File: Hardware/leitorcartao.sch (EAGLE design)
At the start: 167 parts, among them IC1 TL084, IC2 TL084, Q1 BSH103, Q2 BC847ASMD, Q3 BC857ALT1SMD, Q4 BC847ALT1SMD, Q5 BC847ALT1SMD, Q6 BC847ALT1SMD, Q7 BC847ALT1SMD, U1 SAMD20E14A-AUT, U3 TLV1117-50CDCYR, U4 MFRC52202HN1, U5 LP2985-33DBVR, X1 ANTENA 125kHz, X2 MIFARE ANTENA

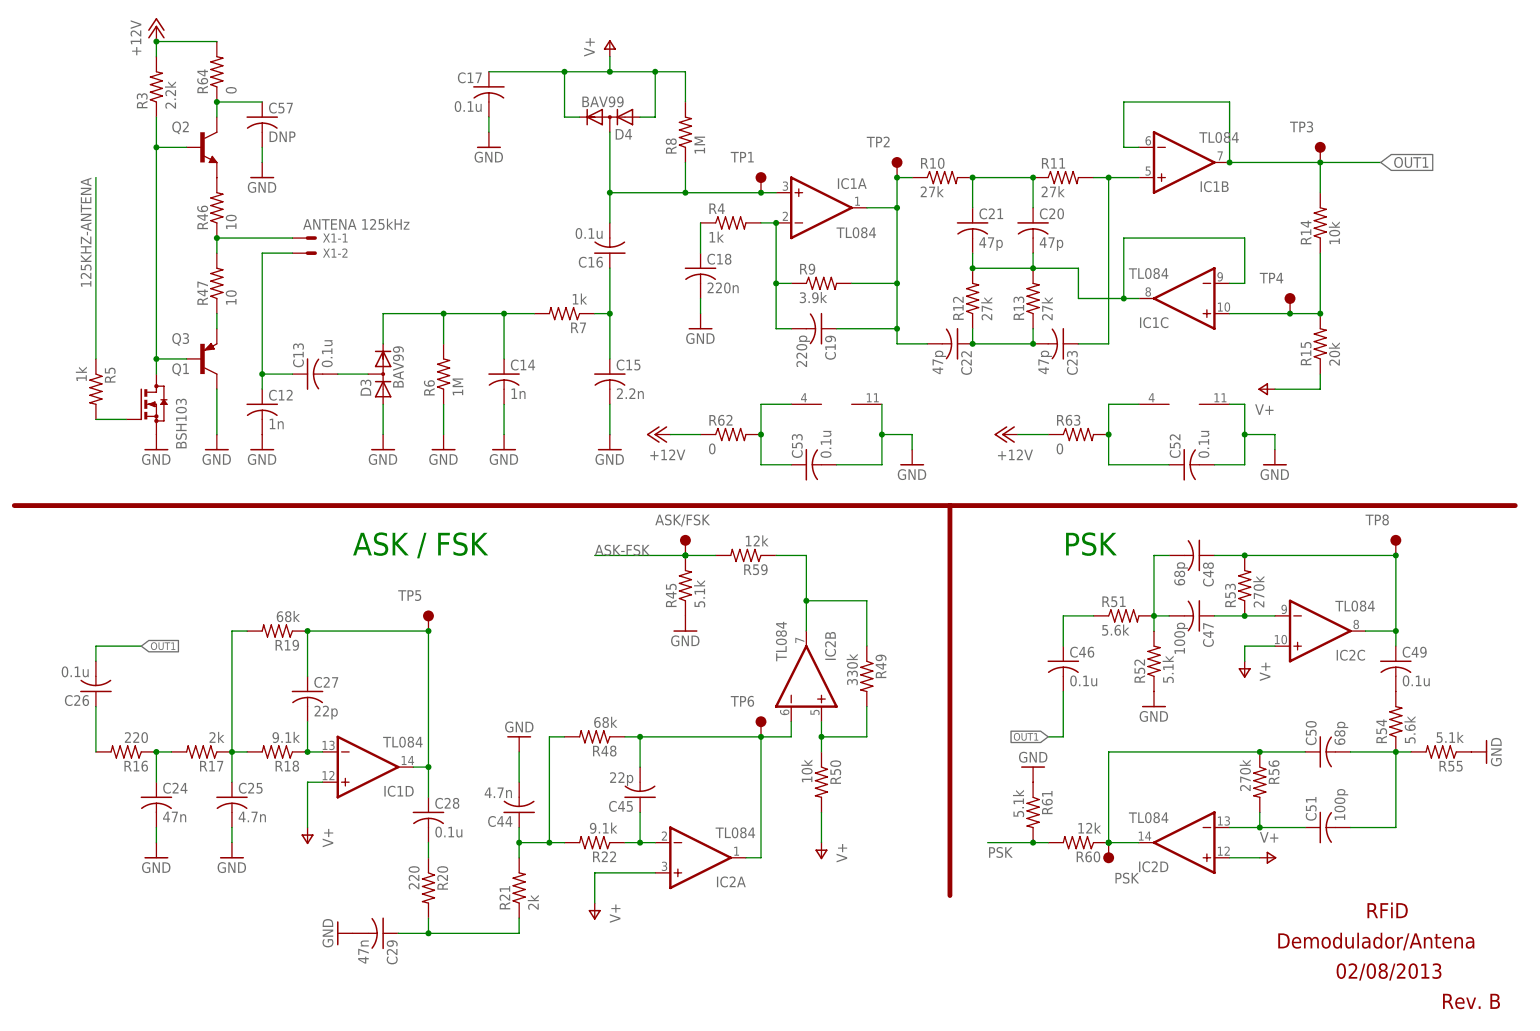
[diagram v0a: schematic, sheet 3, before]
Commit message: Início da versão 3.0
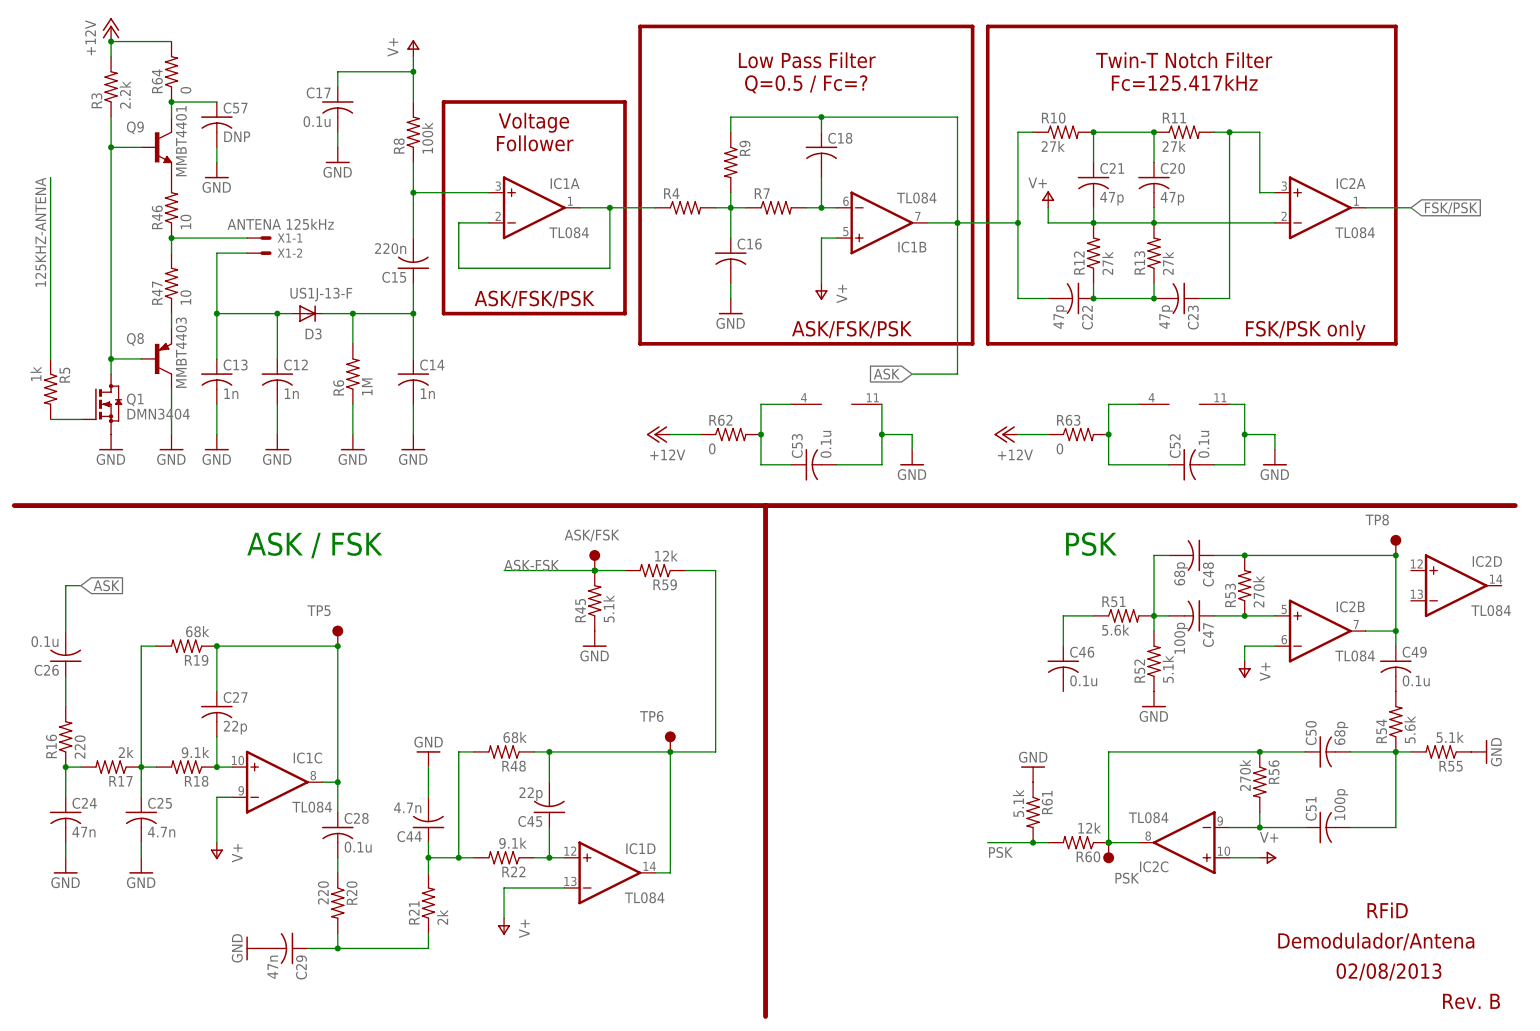
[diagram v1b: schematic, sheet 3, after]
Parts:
- removed C19: 220p, RFiD:C-USC0402
- removed D4: BAV99, RFiD:BAV99
- removed Q2: BC847ASMD, RFiD:BC847ASMD
- removed Q3: BC857ALT1SMD, RFiD:BC857ALT1SMD
- removed R14, R50: 10k, RFiD:R-US_R0402
- removed R15: 20k, RFiD:R-US_R0402
- removed R49: 330k, RFiD:R-US_R0402
- removed TP1, TP2, TP3, TP4: TESTPOINT, RFiD:TESTPOINT
- added Q8: MMBT4403, RFiD:MMBT4403
- added Q9: MMBT4401, RFiD:MMBT4401
- C12: device RFiD:C-USC0603 -> RFiD:C-USC1812; CUSTOMER_PN C/1n/100V/C04 -> (none)
- C13: value 0.1u -> 1n; device RFiD:C-USC0603 -> RFiD:C-USC1206; CUSTOMER_PN C/0.1u/50V/C04 -> (none)
- C14: device RFiD:C-USC0603 -> RFiD:C-USC1206
- C15: value 2.2n -> 220n; device RFiD:C-USC0603 -> RFiD:C-USC1206; CUSTOMER_PN C/2.2n/100V/D04 -> (none)
- C16: value 0.1u -> (none); device RFiD:C-USC0603 -> RFiD:C-USC0402; CUSTOMER_PN C/0.1u/50V/C04 -> C/2.2n/100V/D04
- C18: value 220n -> (none)
- D3: value BAV99 -> US1J-13-F; device RFiD:BAV99 -> RFiD:US1J-13-F
- Q1: value BSH103 -> DMN3404; device RFiD:BSS123 -> RFiD:DMN3404; CUSTOMER_PN Q/BSH103 -> (none)
- R4: value 1k -> (none)
- R6: device RFiD:R-US_R0603 -> RFiD:R-US_R1206
- R7: value 1k -> (none); device RFiD:R-US_R0603 -> RFiD:R-US_R0402; CUSTOMER_PN R/1k/5%/04 -> R/1M/5%/04
- R8: value 1M -> 100k
- R9: value 3.9k -> (none)
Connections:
- removed net N$17: C19.1, C22.2, IC1A.OUT, R10.1, R9.2, TP2.1
- removed net N$21: C20.2, C21.2, IC1C.-IN, IC1C.OUT, R12.2, R13.2
- removed net N$26: IC1C.+IN, R14.1, R15.2, TP4.1
- removed net N$59: Q2.E, R46.2
- removed net N$65: C45.2, IC2A.OUT, IC2B.-IN, R48.1, TP6.1
- removed net N$66: IC2B.+IN, R49.2, R50.1
- removed net OUT1: C26.2, C46.2, IC1B.-IN, IC1B.OUT, R14.2, TP3.1
- new net ASK: C18.1, C22.2, C26.2, IC1B.OUT, R10.1, R9.1
- new net FSK/PSK: IC2A.OUT
- net GND: now also C13.2, C16.2, Q8.C; no longer C15.2, C18.2, D3.1, Q3.C
- net N$10: now also IC1A.-IN, IC1A.OUT; no longer C18.1
- net N$12: now also C16.1, R4.2, R7.1, R9.2; no longer C13.2, D3.3
- net N$13: now also C15.1, D3.K; no longer D3.2, R7.2
- net N$14: now also C15.2, IC1A.+IN, R8.1; no longer C15.1, C16.1, R7.1
- net N$15: now also C18.2, IC1B.-IN, R7.2; no longer C19.2, IC1A.-IN, R4.2, R9.1
- net N$16: now also Q9.E, R46.2; no longer C16.2, D4.3, IC1A.+IN, R8.1, TP1.1
- net N$23: now also IC2A.+IN; no longer IC1B.+IN
- net N$27: now also IC1C.+IN; no longer IC1D.-IN
- net N$28: now also IC1C.OUT; no longer IC1D.OUT
- net N$40: now also IC2C.OUT; no longer IC2D.OUT
- net N$48: now also Q9.C; no longer Q2.C
- net N$60: now also Q8.E; no longer Q3.E
- net N$64: now also IC1D.+IN; no longer IC2A.-IN
- net N$7: now also Q8.B, Q9.B; no longer Q2.B, Q3.B
- net N$71: now also IC2B.OUT; no longer IC2C.OUT
- net N$72: now also IC2B.+IN; no longer IC2C.-IN
- net N$75: now also IC2C.-IN; no longer IC2D.-IN
- net N$9: now also D3.A
- net N$90: now also C45.2, IC1D.OUT, R48.1, TP6.1; no longer IC2B.OUT, R49.1
- net V+: now also C20.2, C21.2, IC1B.+IN, IC1C.-IN, IC1D.-IN, IC2A.-IN, IC2B.-IN, R12.2, R13.2; no longer D4.1, D4.2, IC1D.+IN, IC2A.+IN, IC2D.+IN, R15.1, R50.2
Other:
- note added: "ASK/FSK/PSK"
- note added: "FSK/PSK only"
- note added: "Low Pass Filter Q=0.5 / Fc=?"
- note added: "Twin-T Notch Filter Fc=125.417kHz"
- note added: "Voltage Follower"
- moved on the sheet: ASK/FSK, C12, C13, C14, C15, C16, C17, C18, C20, C21, C22, C23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
